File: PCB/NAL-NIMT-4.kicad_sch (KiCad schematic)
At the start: 19 parts

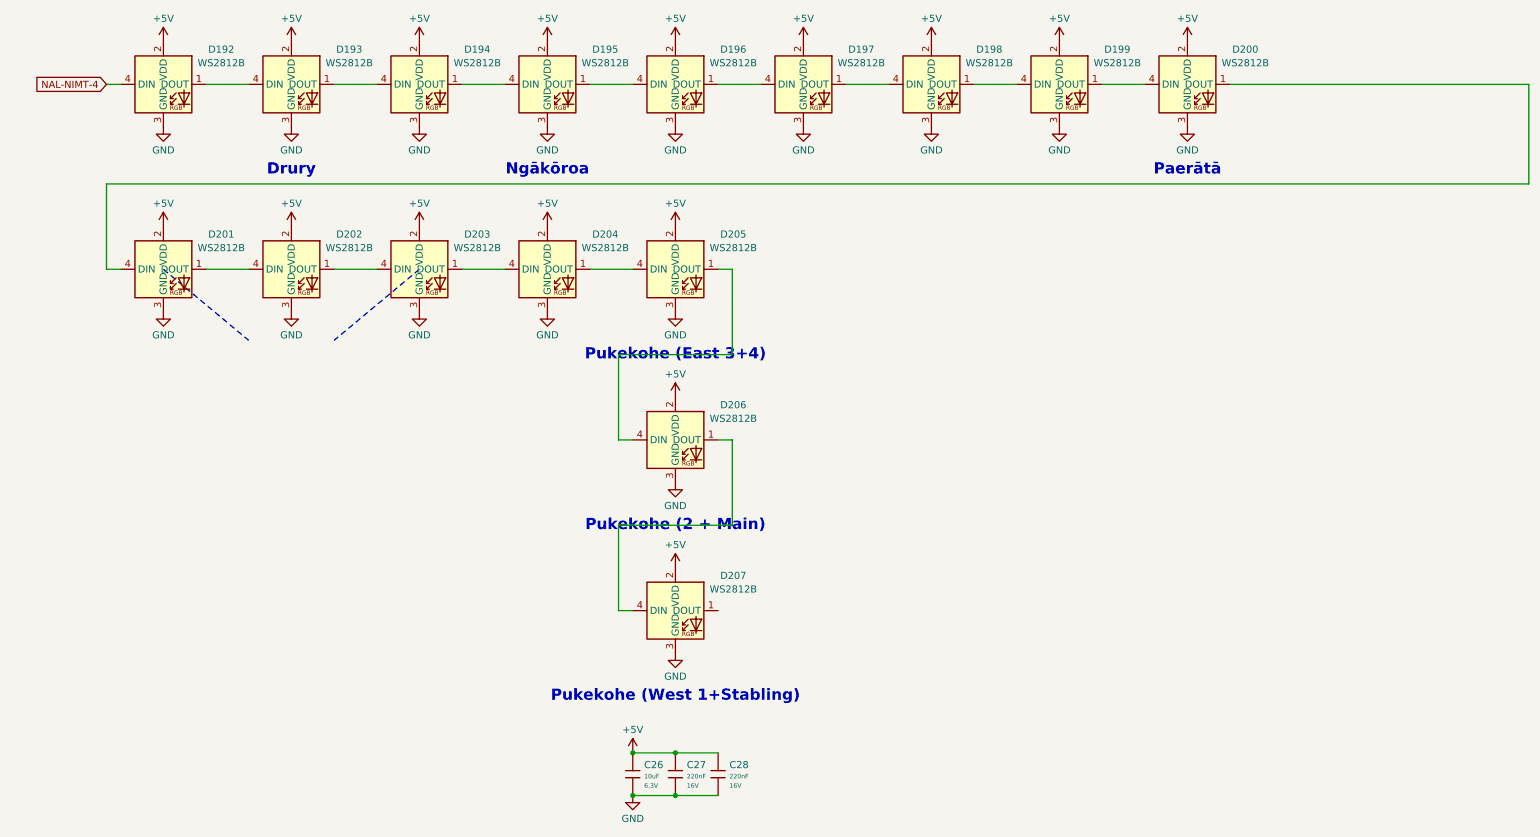
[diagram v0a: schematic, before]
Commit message: Final tweaks for V1.0.0
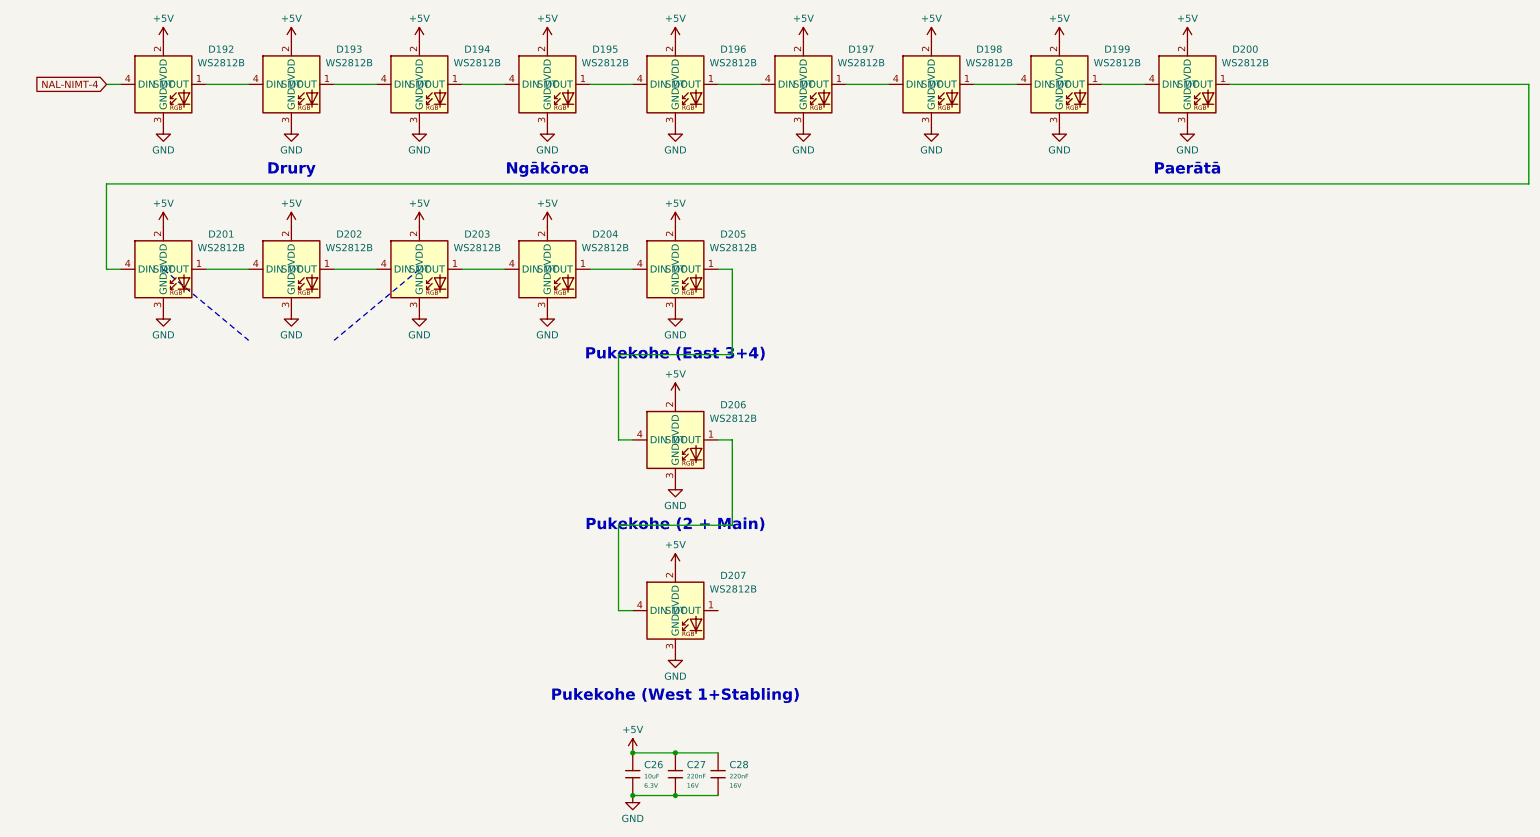
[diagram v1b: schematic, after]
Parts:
- D192, D193, D194, D195, D196, D197, D198, D199, D200, D201, D202, D203, D204, D205, D206, D207: Manufacturer (none) -> XINGLIGHT; Part (none) -> XL-1615RGBC-WS2812B; Process (none) -> SMT
